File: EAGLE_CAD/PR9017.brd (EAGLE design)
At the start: 70 x 70 mm, 72 parts

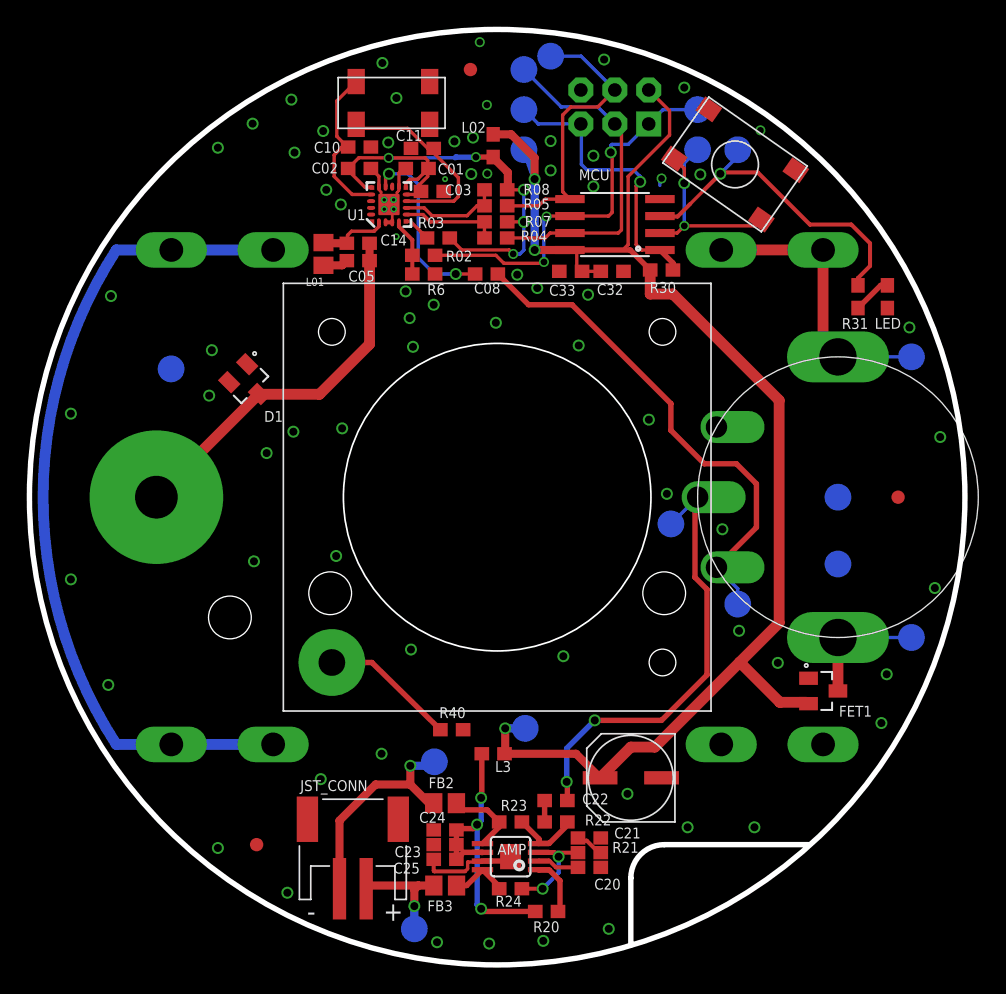
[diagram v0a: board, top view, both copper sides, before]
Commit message: DRC Changes
DRC Changes
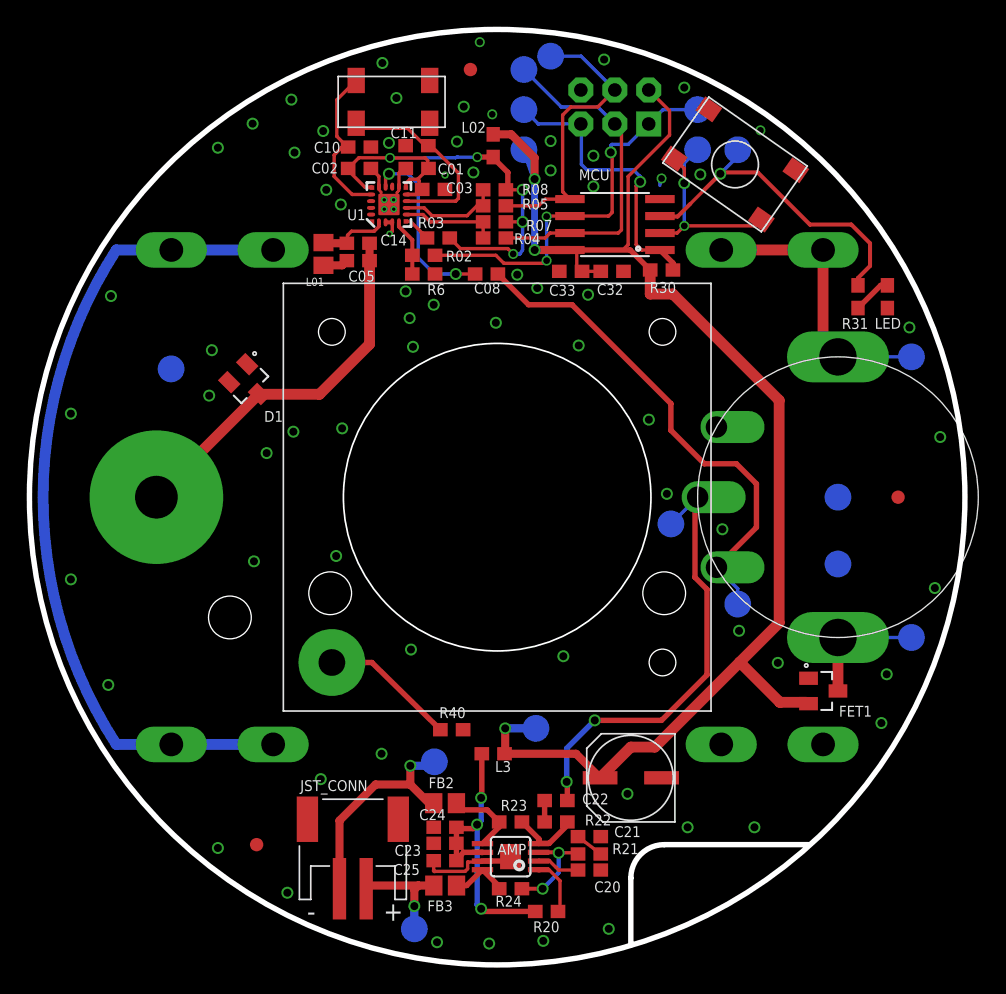
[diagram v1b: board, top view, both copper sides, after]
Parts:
- moved TP4 0.80 mm to (37.9, 17.7)
- moved C11 0.45 mm to (29.0, 61.3)
- moved C24 0.20 mm to (31.1, 10.3)
- moved C20 0.20 mm to (41.9, 7.10)
- moved C03 0.17 mm to (30.2, 58.0)
- moved R04 0.10 mm to (34.8, 54.4)
- moved R05 0.10 mm to (34.8, 56.8)
- moved R07 0.10 mm to (34.8, 55.6)
- moved R08 0.10 mm to (34.8, 58.0)
- moved C25 0.10 mm to (31.1, 7.80)
- moved C21 0.10 mm to (41.9, 9.60)
- moved C23 0.10 mm to (31.1, 9.10)
- moved R21 0.10 mm to (41.9, 8.30)
- moved X1 0.08 mm to (27.2, 64.6)
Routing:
- net N$5: track 9.04 -> 7.77 mm
- net VCC: track 110.9 -> 111.7 mm
- net GND: vias 74 -> 73
